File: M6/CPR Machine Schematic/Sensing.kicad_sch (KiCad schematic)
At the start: 6 parts, among them J12 I2C Port, J8 Force Sensor, U3 MCP6001R

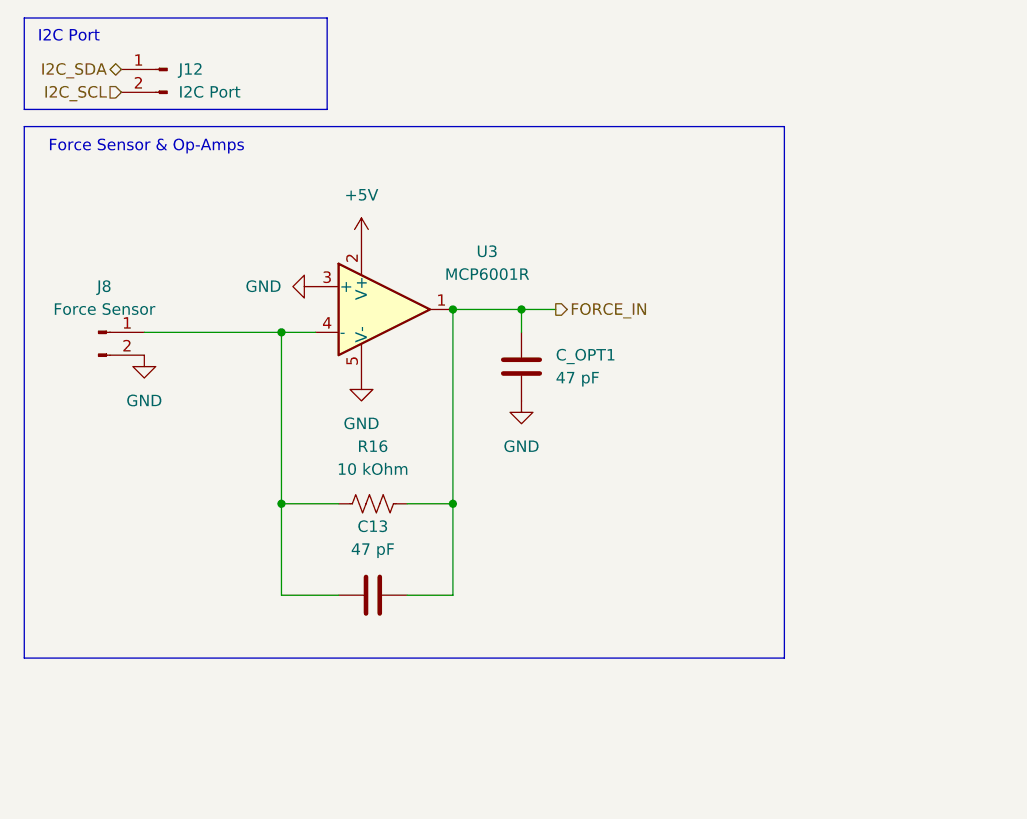
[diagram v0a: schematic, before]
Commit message: PCB Feedback V1
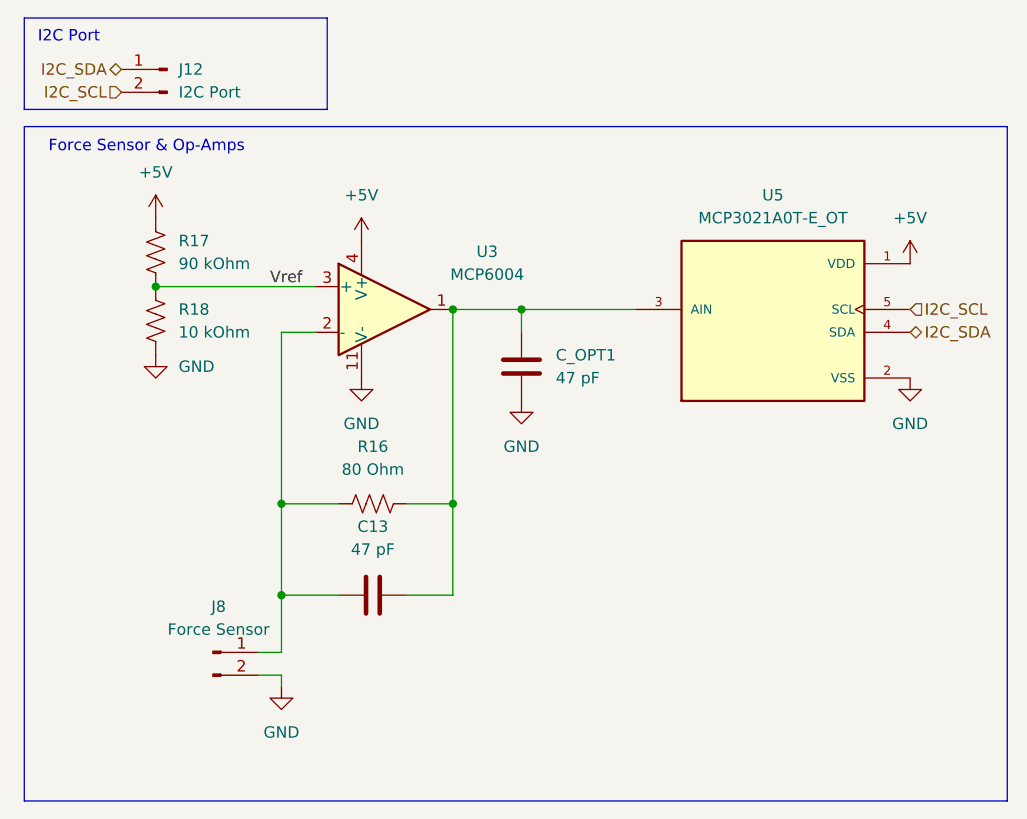
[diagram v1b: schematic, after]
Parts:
- added R17: 90 kOhm, Resistor_SMD:R_1206_3216Metric, symbol Device:R_US
- added R18: 10 kOhm, Resistor_SMD:R_1206_3216Metric, symbol Device:R_US
- added U5: MCP3021A0T-E_OT, 2679:IC_MCP3021A0T-E_OT, symbol Custom_Parts:MCP3021A0T-E_OT
- R16: value 10 kOhm -> 80 Ohm
- U3: value MCP6001R -> MCP6004; footprint Package_TO_SOT_SMD:SOT-23-5 -> MCP6004:SOIC14_SL_MCH
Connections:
- net +5V: now also U3.4 (V+), R17.1, U5.1 (VDD); no longer U3.2 (V+)
- net GND: now also U3.11 (V-), R18.2, U5.2 (VSS); no longer U3.3 (+), U3.5 (V-)
- net I2C_SCL: now also U5.5 (SCL)
- net I2C_SDA: now also U5.4 (SDA)
- net at C13.1, J8.1 (Pin_1), R16.2: now also U3.2 (-); no longer U3.4 (-)
- net FORCE_IN: no longer names the net of C13.2, C_OPT1.2, R16.1, U3.1
- net FORCE_IN: now also U5.3 (AIN)
- new net Vref: R17.2, R18.1, U3.3 (+)
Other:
- moved on the sheet: J8
